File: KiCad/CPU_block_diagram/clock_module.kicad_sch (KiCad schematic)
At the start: 6 parts, among them U1 LM555xN

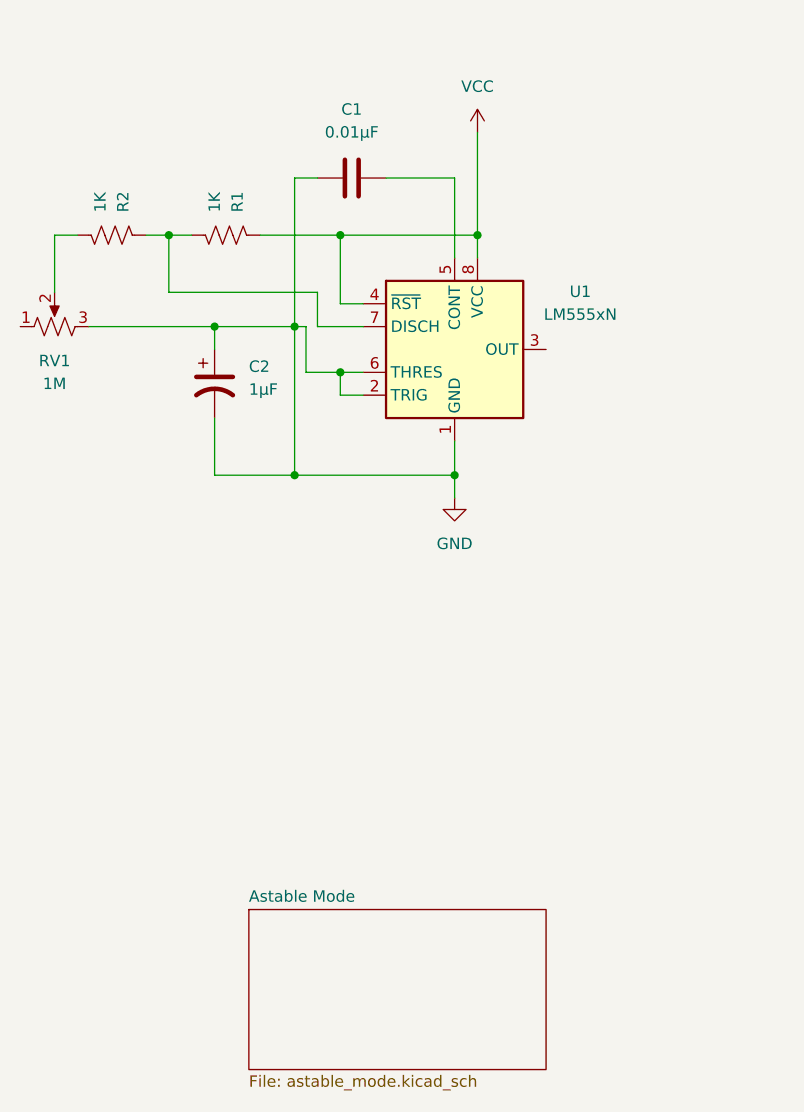
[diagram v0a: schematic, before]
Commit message: vault backup: 2025-12-29 00:49:08
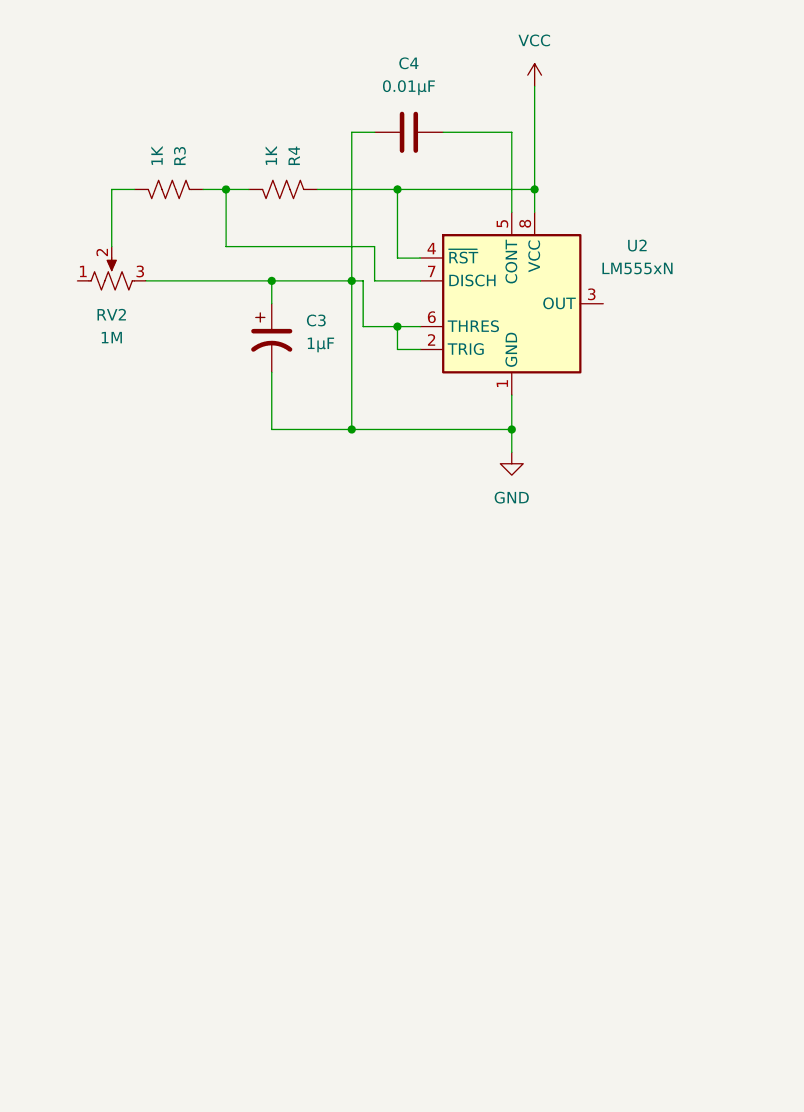
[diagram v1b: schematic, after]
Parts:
- removed C1: 0.01µF, symbol Device:C
- removed C2: 1µF, symbol Device:C_Polarized_US
- removed R1, R2: 1K, symbol Device:R_US
- removed RV1: 1M, symbol Device:R_Potentiometer_US
- removed U1: LM555xN, Package_DIP:DIP-8_W7.62mm, symbol Timer:LM555xN
- added C3: 1µF, symbol Device:C_Polarized_US
- added C4: 0.01µF, symbol Device:C
- added R3, R4: 1K, symbol Device:R_US
- added RV2: 1M, symbol Device:R_Potentiometer_US
- added U2: LM555xN, Package_DIP:DIP-8_W7.62mm, symbol Timer:LM555xN
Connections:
- net GND: now also C3.1, C3.2, C4.1, RV2.3, U2.1 (GND), U2.2 (TRIG), U2.6 (THRES)
- net VCC: now also R4.1, U2.4 (~{RST}), U2.8 (VCC)
- new net: R3.1, R4.2, U2.7 (DISCH)
- new net: C4.2, U2.5 (CONT)
- new net: R3.2, RV2.2
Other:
- removed sheet Astable Mode

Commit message: vault backup: 2025-12-29 04:12:58
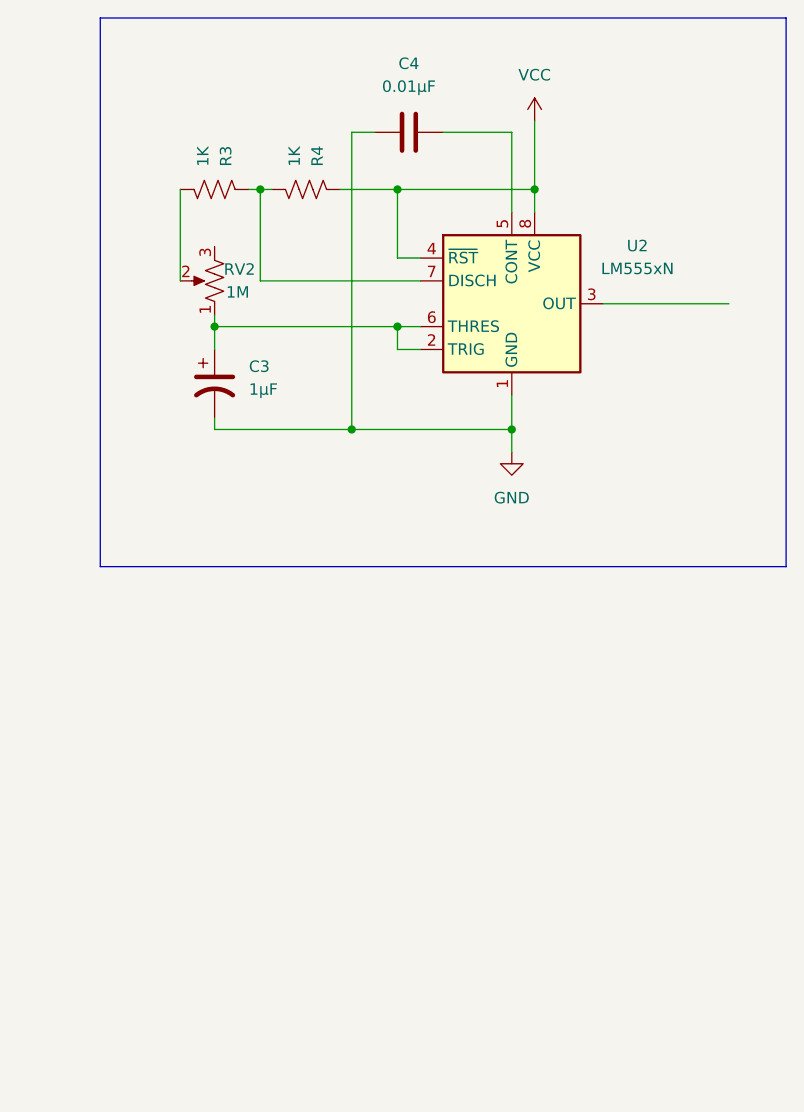
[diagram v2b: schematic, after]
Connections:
- net GND: no longer C3.1, RV2.3, U2.2 (TRIG), U2.6 (THRES)
- net at RV2.1: now also C3.1, U2.2 (TRIG), U2.6 (THRES)
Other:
- moved on the sheet: C3, R3, R4, RV2
